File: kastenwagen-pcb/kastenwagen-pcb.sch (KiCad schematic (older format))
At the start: 9 parts

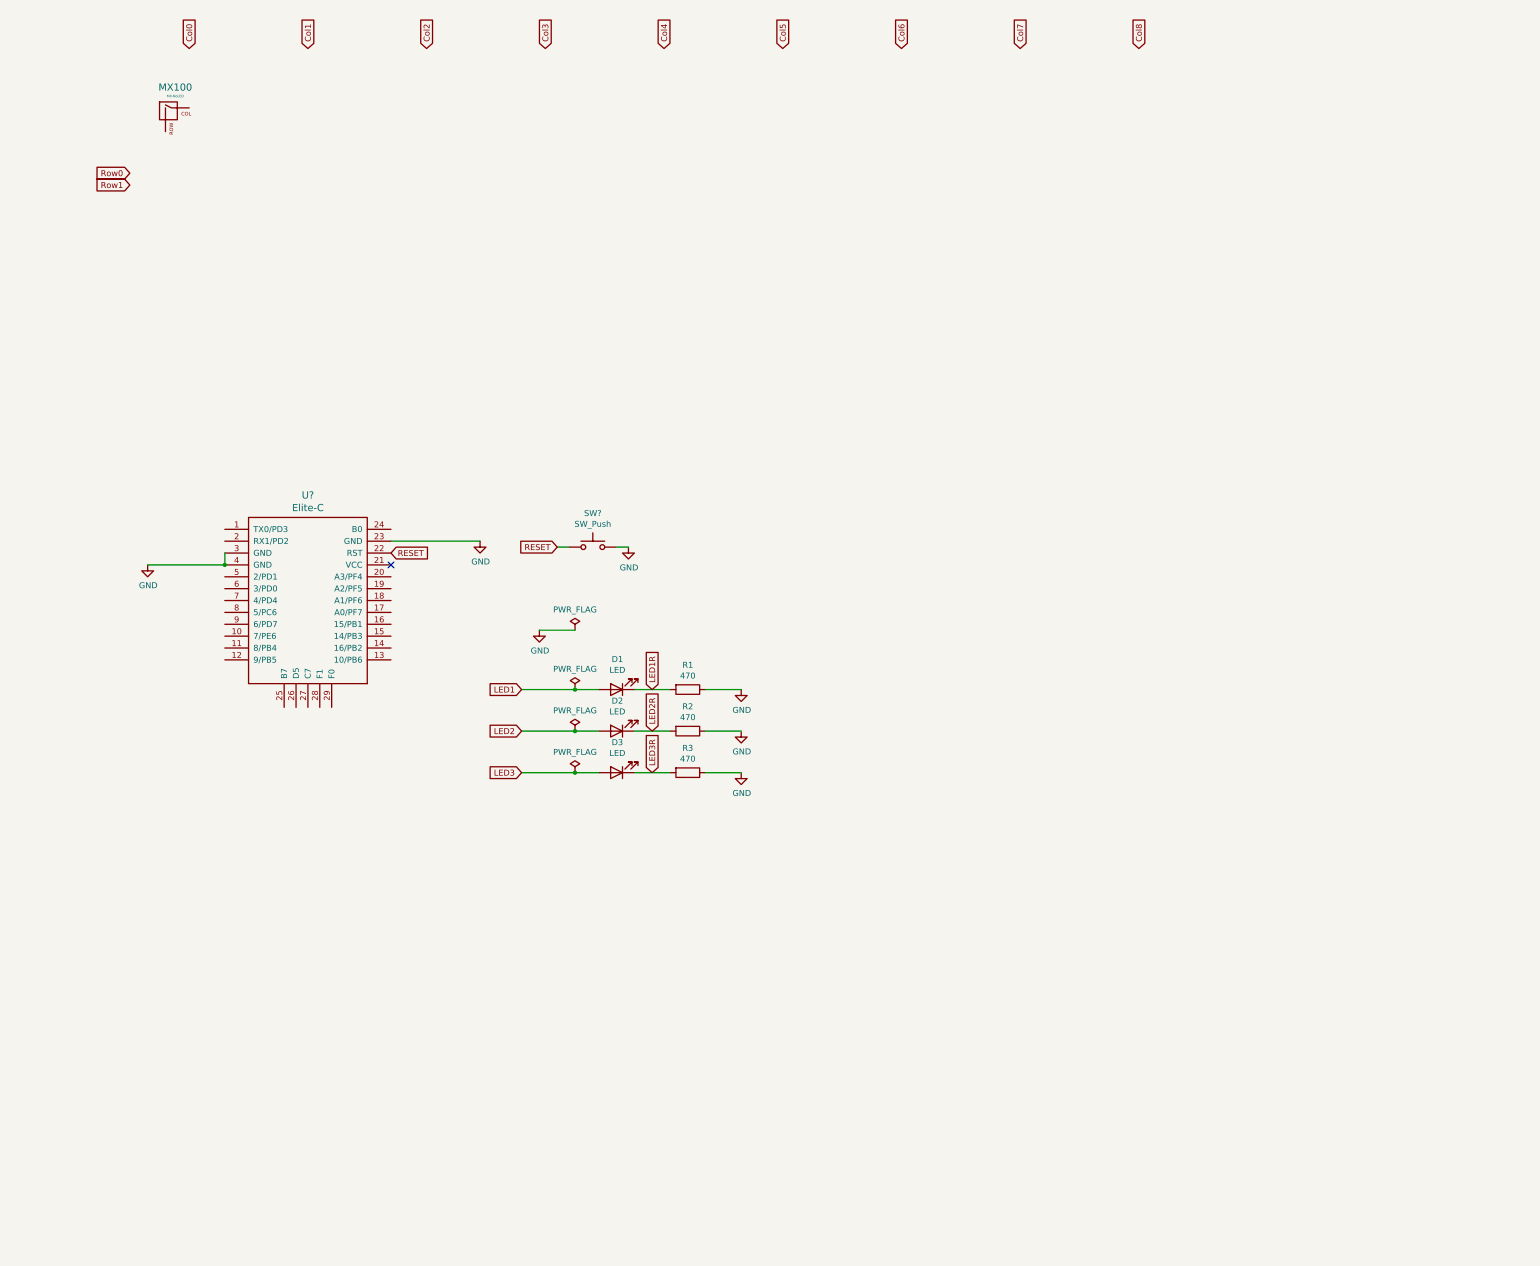
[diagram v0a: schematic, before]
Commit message: Complete Schema
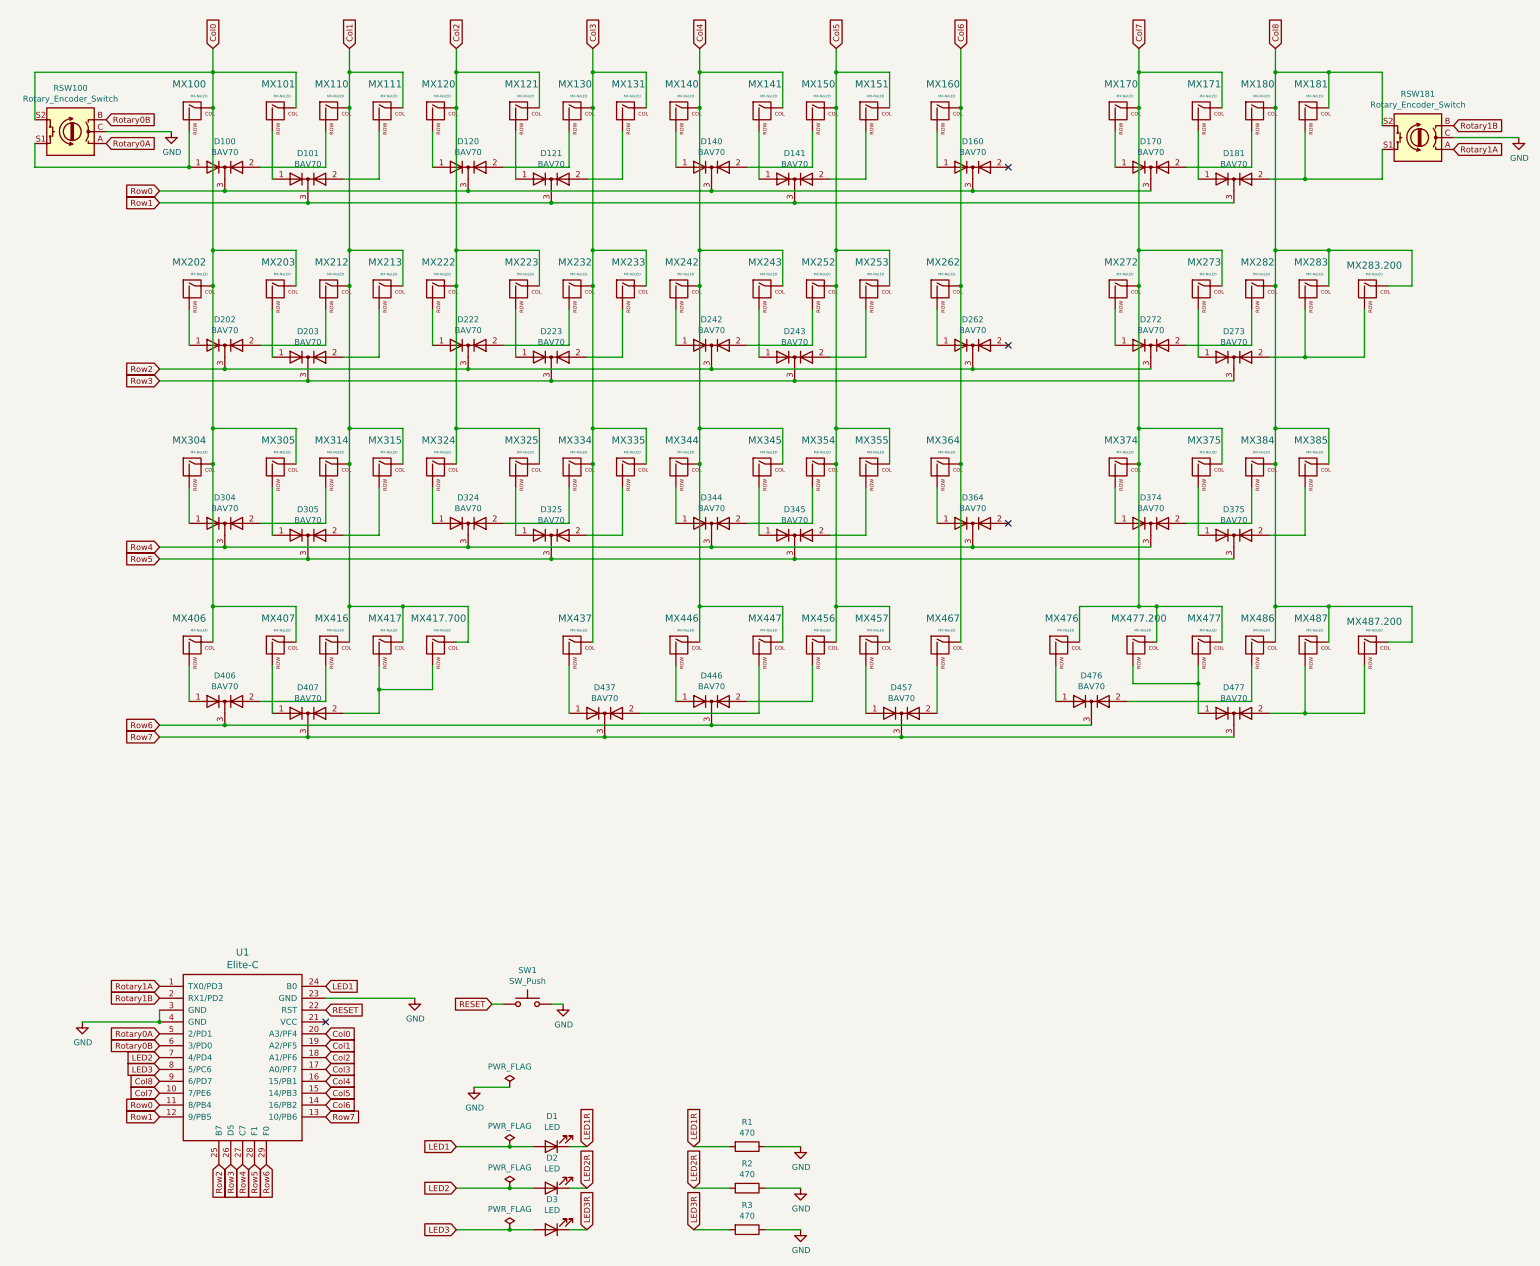
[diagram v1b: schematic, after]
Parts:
- added D100, D101, D120, D121, D140, D141, D160, D170, D181, D202, D203, D222, D223, D242, D243, D262, D272, D273, D304, D305, D324, D325, D344, D345, D364, D374, D375, D406, D407, D437, D446, D457, D476, D477: BAV70, Keebio-Parts:SOT-23_Handsoldering, symbol Diode:BAV70
- added MX101, MX110, MX111, MX120, MX121, MX130, MX131, MX140, MX141, MX150, MX151, MX170, MX171, MX180, MX181, MX203, MX212, MX213, MX222, MX223, MX232, MX233, MX242, MX243, MX252, MX253, MX272, MX273, MX282, MX283, MX305, MX314, MX315, MX324, MX325, MX334, MX335, MX344, MX345, MX354, MX364, MX374, MX375, MX384, MX385, MX416, MX446, MX457, MX467, MX476, MX477, MX486, MX487: MX-NoLED, MX_Only:MXOnly-1U-NoLED, symbol MX_Alps_Hybrid:MX-NoLED
- added MX160, MX304: MX-NoLED, MX_Only:MXOnly-1.75U-NoLED, symbol MX_Alps_Hybrid:MX-NoLED
- added MX202, MX355, MX406, MX407, MX447, MX456: MX-NoLED, MX_Only:MXOnly-1.25U-NoLED, symbol MX_Alps_Hybrid:MX-NoLED
- added MX262: MX-NoLED, MX_Only:MXOnly-1.5U-NoLED, symbol MX_Alps_Hybrid:MX-NoLED
- added MX283.200, MX487.200: MX-NoLED, MX_Only:MXOnly-2U-ReversedStabilizers-NoLED, symbol MX_Alps_Hybrid:MX-NoLED
- added MX417: MX-NoLED, MX_Only:MXOnly-2.75U-NoLED, symbol MX_Alps_Hybrid:MX-NoLED
- added MX417.700: MX-NoLED, MX_Only:MXOnly-7U-NoLED, symbol MX_Alps_Hybrid:MX-NoLED
- added MX437: MX-NoLED, MX_Only:MXOnly-2.25U-NoLED, symbol MX_Alps_Hybrid:MX-NoLED
- added MX477.200: MX-NoLED, MX_Only:MXOnly-2U-NoLED, symbol MX_Alps_Hybrid:MX-NoLED
- added RSW100, RSW181: Rotary_Encoder_Switch, Keebio-Parts:RotaryEncoder_Alps_EC11E-Switch_Vertical_H20mm, symbol Device:Rotary_Encoder_Switch
- D1, D2, D3: footprint (none) -> LED_THT:LED_D3.0mm
- MX100: footprint (none) -> MX_Only:MXOnly-1U-NoLED
- R1, R2, R3: footprint (none) -> Keebio-Parts:Resistor-Hybrid-Back
- SW1: renamed from SW?; footprint (none) -> Keebio-Parts:SW_Tactile_SPST_Angled_MJTP1117
- U1: renamed from U?; footprint (none) -> Keebio-Parts:Elite-C-castellated-29pin-holes
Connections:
- net Col0: now also MX100.1 (COL), U1.20 (A3/PF4), MX101.1 (COL), MX202.1 (COL), MX203.1 (COL), MX304.1 (COL), MX305.1 (COL), MX406.1 (COL), MX407.1 (COL), RSW100.S2
- net Col1: now also U1.19 (A2/PF5), MX110.1 (COL), MX111.1 (COL), MX212.1 (COL), MX213.1 (COL), MX314.1 (COL), MX315.1 (COL), MX416.1 (COL), MX417.1 (COL), MX417.700.1 (COL)
- net Col2: now also U1.18 (A1/PF6), MX120.1 (COL), MX121.1 (COL), MX222.1 (COL), MX223.1 (COL), MX324.1 (COL), MX325.1 (COL)
- net Col3: now also U1.17 (A0/PF7), MX130.1 (COL), MX131.1 (COL), MX232.1 (COL), MX233.1 (COL), MX334.1 (COL), MX335.1 (COL), MX437.1 (COL)
- net Col4: now also U1.16 (15/PB1), MX140.1 (COL), MX141.1 (COL), MX242.1 (COL), MX243.1 (COL), MX344.1 (COL), MX345.1 (COL), MX446.1 (COL), MX447.1 (COL)
- net Col5: now also U1.15 (14/PB3), MX150.1 (COL), MX151.1 (COL), MX252.1 (COL), MX253.1 (COL), MX354.1 (COL), MX355.1 (COL), MX456.1 (COL), MX457.1 (COL)
- net Col6: now also U1.14 (16/PB2), MX160.1 (COL), MX262.1 (COL), MX364.1 (COL), MX467.1 (COL)
- net Col7: now also U1.10 (7/PE6), MX170.1 (COL), MX171.1 (COL), MX272.1 (COL), MX273.1 (COL), MX374.1 (COL), MX375.1 (COL), MX476.1 (COL), MX477.1 (COL), MX477.200.1 (COL)
- net Col8: now also U1.9 (6/PD7), MX180.1 (COL), MX181.1 (COL), MX282.1 (COL), MX283.1 (COL), MX283.200.1 (COL), MX384.1 (COL), MX385.1 (COL), MX486.1 (COL), MX487.1 (COL), MX487.200.1 (COL), RSW181.S2
- net GND: now also RSW100.C, RSW181.C
- net LED1: now also U1.24 (B0)
- net LED2: now also U1.7 (4/PD4)
- net LED3: now also U1.8 (5/PC6)
- net Row0: now also U1.11 (8/PB4), D100.3 (K), D120.3 (K), D140.3 (K), D160.3 (K), D170.3 (K)
- net Row1: now also U1.12 (9/PB5), D101.3 (K), D121.3 (K), D141.3 (K), D181.3 (K)
- net Rotary1A: now reaches U1.1 (TX0/PD3)
- net Rotary1A: now also RSW181.A
- net Row7: now reaches U1.13 (10/PB6)
- net Row7: now also D407.3 (K), D437.3 (K), D457.3 (K), D477.3 (K)
- net Rotary1B: now reaches U1.2 (RX1/PD2)
- net Rotary1B: now also RSW181.B
- net Row2: now reaches U1.25 (B7)
- net Row2: now also D202.3 (K), D222.3 (K), D242.3 (K), D262.3 (K), D272.3 (K)
- net Row3: now reaches U1.26 (D5)
- net Row3: now also D203.3 (K), D223.3 (K), D243.3 (K), D273.3 (K)
- net Row4: now reaches U1.27 (C7)
- net Row4: now also D304.3 (K), D324.3 (K), D344.3 (K), D364.3 (K), D374.3 (K)
- net Row5: now reaches U1.28 (F1)
- net Row5: now also D305.3 (K), D325.3 (K), D345.3 (K), D375.3 (K)
- net Row6: now reaches U1.29 (F0)
- net Row6: now also D406.3 (K), D446.3 (K), D476.3 (K)
- net Rotary0A: now reaches U1.5 (2/PD1)
- net Rotary0A: now also RSW100.A
- net Rotary0B: now reaches U1.6 (3/PD0)
- net Rotary0B: now also RSW100.B
- net at MX100.2 (ROW): now also D100.1 (A), RSW100.S1
- new net: D101.1 (A), MX101.2 (ROW)
- new net: D100.2 (A), MX110.2 (ROW)
- new net: D101.2 (A), MX111.2 (ROW)
- new net: D120.1 (A), MX120.2 (ROW)
- new net: D121.1 (A), MX121.2 (ROW)
- new net: D120.2 (A), MX130.2 (ROW)
- new net: D121.2 (A), MX131.2 (ROW)
- new net: D140.1 (A), MX140.2 (ROW)
- new net: D141.1 (A), MX141.2 (ROW)
- new net: D140.2 (A), MX150.2 (ROW)
- new net: D141.2 (A), MX151.2 (ROW)
- new net: D160.1 (A), MX160.2 (ROW)
- new net: D170.1 (A), MX170.2 (ROW)
- new net: D181.1 (A), MX171.2 (ROW)
- new net: D170.2 (A), MX180.2 (ROW)
- new net: D181.2 (A), MX181.2 (ROW), RSW181.S1
- new net: D202.1 (A), MX202.2 (ROW)
- new net: D203.1 (A), MX203.2 (ROW)
- new net: D202.2 (A), MX212.2 (ROW)
- new net: D203.2 (A), MX213.2 (ROW)
- new net: D222.1 (A), MX222.2 (ROW)
- new net: D223.1 (A), MX223.2 (ROW)
- new net: D222.2 (A), MX232.2 (ROW)
- new net: D223.2 (A), MX233.2 (ROW)
- new net: D242.1 (A), MX242.2 (ROW)
- new net: D243.1 (A), MX243.2 (ROW)
- new net: D242.2 (A), MX252.2 (ROW)
- new net: D243.2 (A), MX253.2 (ROW)
- new net: D262.1 (A), MX262.2 (ROW)
- new net: D272.1 (A), MX272.2 (ROW)
- new net: D273.1 (A), MX273.2 (ROW)
- new net: D272.2 (A), MX282.2 (ROW)
- new net: D273.2 (A), MX283.2 (ROW), MX283.200.2 (ROW)
- new net: D304.1 (A), MX304.2 (ROW)
- new net: D305.1 (A), MX305.2 (ROW)
- new net: D304.2 (A), MX314.2 (ROW)
- new net: D305.2 (A), MX315.2 (ROW)
- new net: D324.1 (A), MX324.2 (ROW)
- new net: D325.1 (A), MX325.2 (ROW)
- new net: D324.2 (A), MX334.2 (ROW)
- new net: D325.2 (A), MX335.2 (ROW)
- new net: D344.1 (A), MX344.2 (ROW)
- new net: D345.1 (A), MX345.2 (ROW)
- new net: D344.2 (A), MX354.2 (ROW)
- new net: D345.2 (A), MX355.2 (ROW)
- new net: D364.1 (A), MX364.2 (ROW)
- new net: D374.1 (A), MX374.2 (ROW)
- new net: D375.1 (A), MX375.2 (ROW)
- new net: D374.2 (A), MX384.2 (ROW)
- new net: D375.2 (A), MX385.2 (ROW)
- new net: D406.1 (A), MX406.2 (ROW)
- new net: D407.1 (A), MX407.2 (ROW)
- new net: D406.2 (A), MX416.2 (ROW)
- new net: D407.2 (A), MX417.2 (ROW), MX417.700.2 (ROW)
- new net: D437.1 (A), MX437.2 (ROW)
- new net: D437.2 (A), MX447.2 (ROW)
- new net: D446.1 (A), MX446.2 (ROW)
- new net: D446.2 (A), MX456.2 (ROW)
- new net: D457.1 (A), MX457.2 (ROW)
- new net: D457.2 (A), MX467.2 (ROW)
- new net: D476.1 (A), MX476.2 (ROW)
- new net: D477.1 (A), MX477.2 (ROW), MX477.200.2 (ROW)
- new net: D476.2 (A), MX486.2 (ROW)
- new net: D477.2 (A), MX487.2 (ROW), MX487.200.2 (ROW)
- no-connect marks 1 -> 4
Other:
- moved on the sheet: D1, D2, D3, MX100, SW1, U1
